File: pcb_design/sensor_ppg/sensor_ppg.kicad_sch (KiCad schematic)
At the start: 12 parts, among them J1 Conn_01x07_Pin, U1 MAX30102EFD_T, U2 MIC5365-1.8YMT-TZ

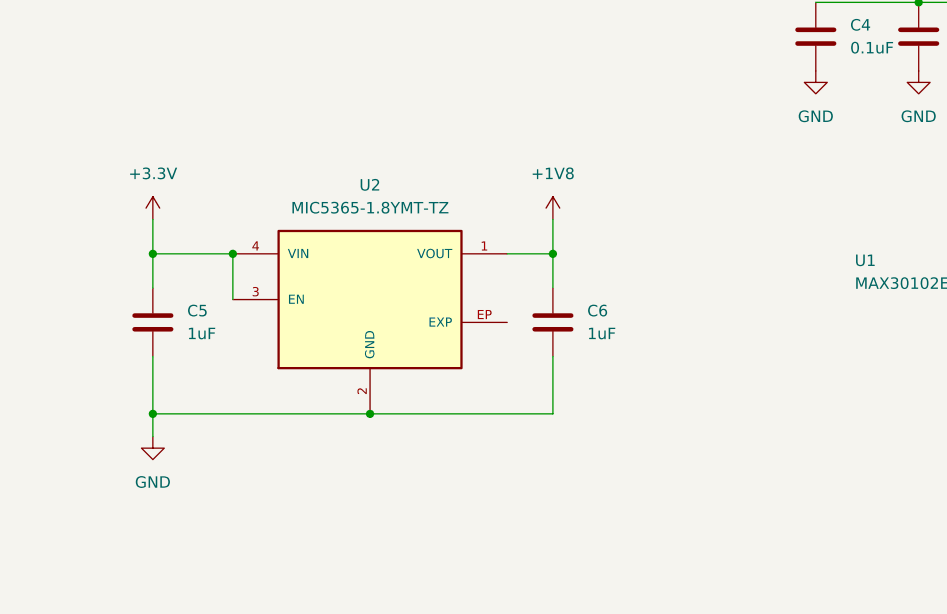
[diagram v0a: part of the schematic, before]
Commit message: update pcb, cad, and code
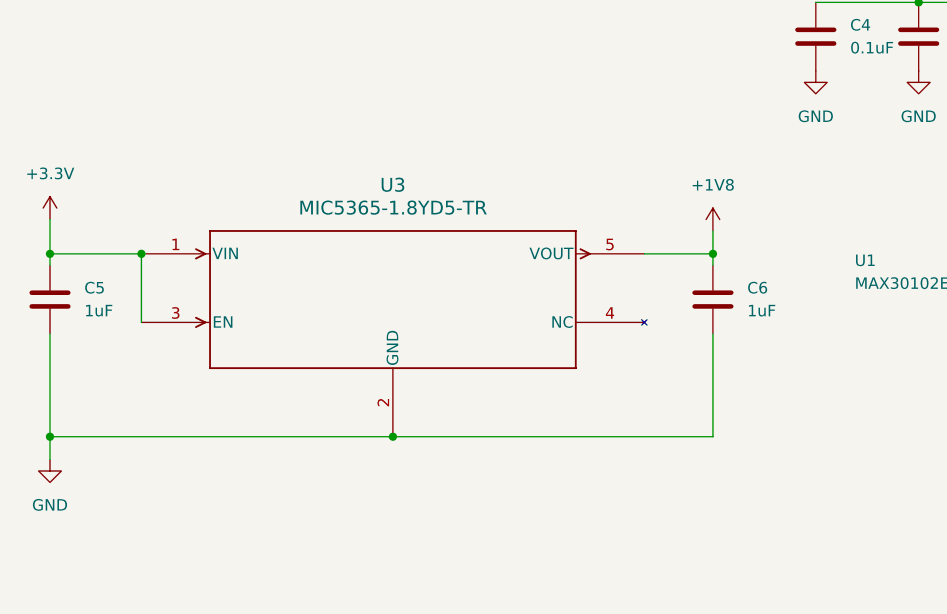
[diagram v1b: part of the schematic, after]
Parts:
- removed U2: MIC5365-1.8YMT-TZ, MIC5365_1_8YMT_TZ_snap:VREG_MIC5365-1.8YMT-TZ, symbol MIC5365-1.8YMT-TZ_snap:MIC5365-1.8YMT-TZ
- added U3: MIC5365-1.8YD5-TR, MIC5365_1_8YD5_TR:TSOT-23-5_D5_MCH, symbol MIC5365_1_8YD5_TR:MIC5365-1.8YD5-TR
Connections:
- net +1V8: now also U3.5 (VOUT)
- net +3.3V: now also U3.1 (VIN), U3.3 (EN)
- net GND: now also U3.2 (GND)
